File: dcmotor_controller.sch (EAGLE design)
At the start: 72 parts, among them IC1 L298, IC2 L298, IC3 AS5040, IC5 SN74LVCR162245A, Q1 8MHz, U1 STM32F051C8T6

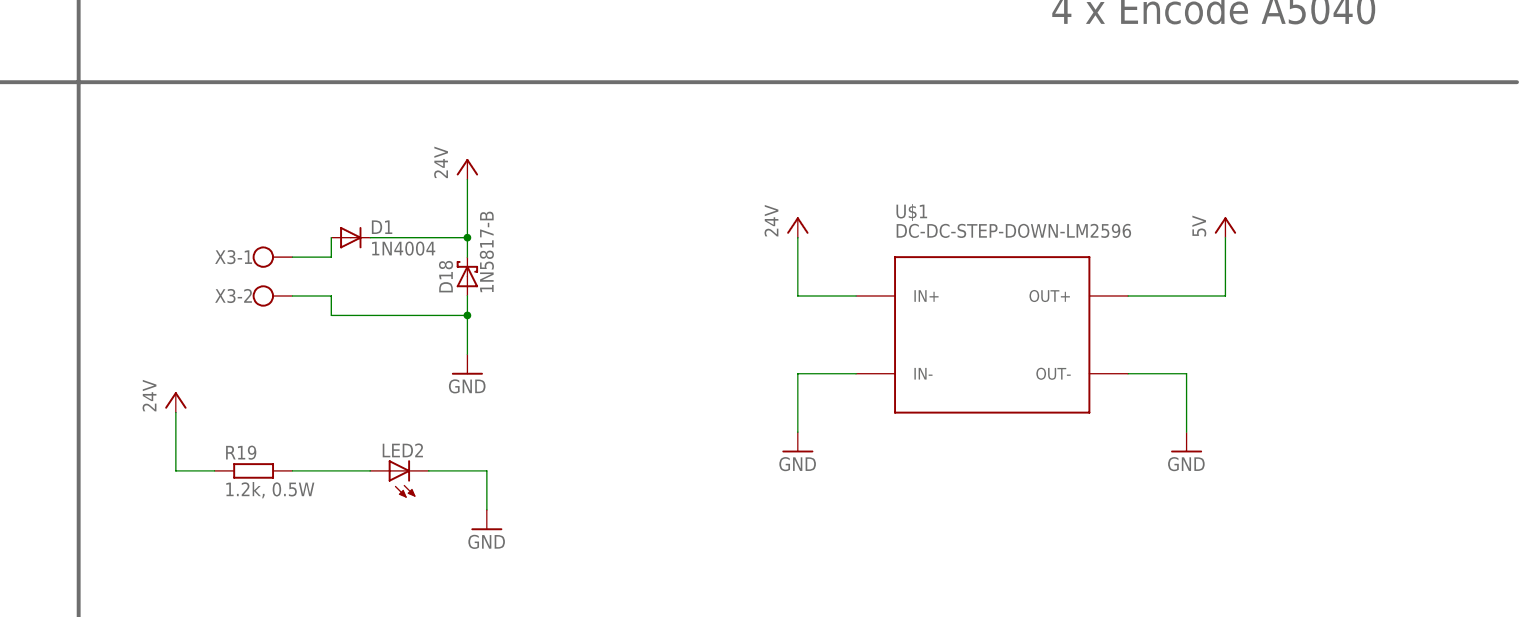
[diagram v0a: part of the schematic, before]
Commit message: poprawione zasilanie
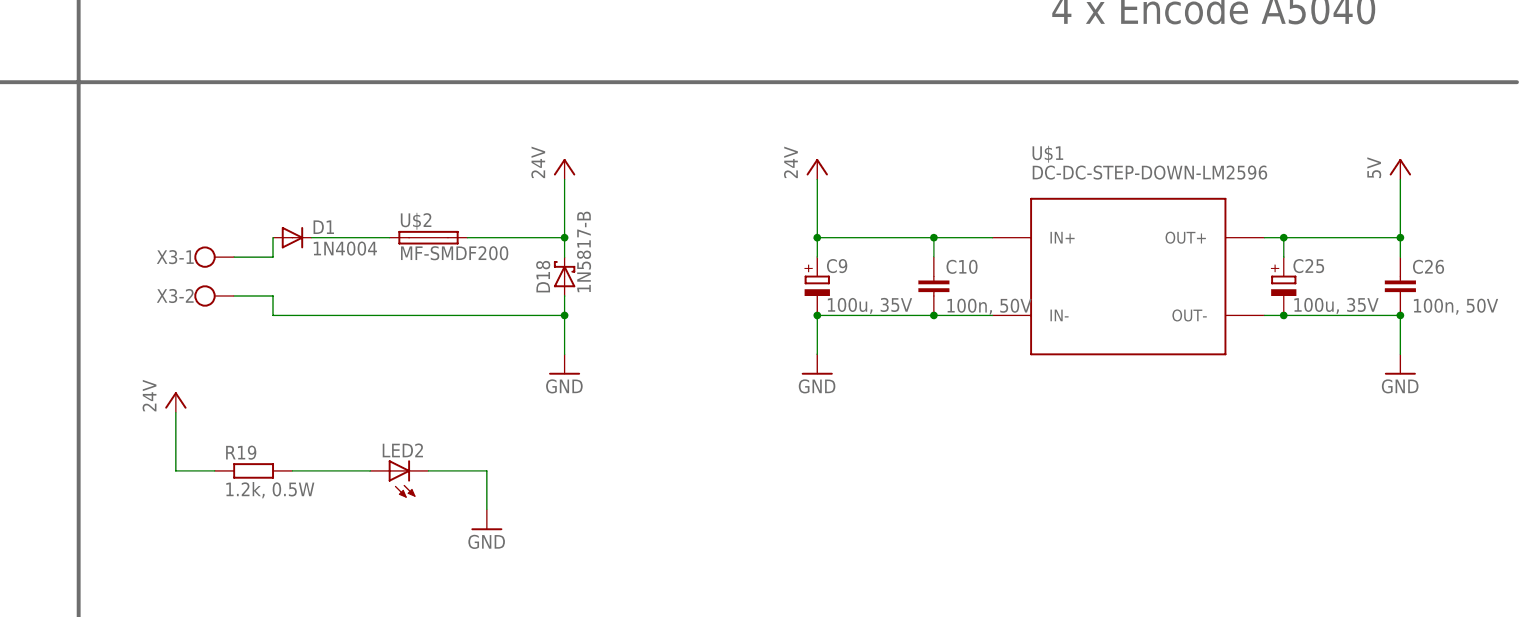
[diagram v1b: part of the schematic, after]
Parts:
- added C10, C26: 100n, 50V, rcl:C-EU025-025X050
- added C25, C9: 100u, 35V, rcl:CPOL-EUD
- added U$2: MF-SMDF200, fuse:MF-SMDF200
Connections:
- new net N$12: D1.C, U$2.1
- net GND: now also C10.2, C25.-, C26.2, C9.-
- net VCC: now also C10.1, C25.+, C26.1, C9.+, U$2.2; no longer D1.C
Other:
- moved on the sheet: D1, D18, U$1, X3-1, X3-2
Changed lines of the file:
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@@
 <part name="GND47" library="supply1" library_urn="urn:adsk.eagle:library:371" deviceset="GND" device=""/>
 <part name="P+5" library="supply1" library_urn="urn:adsk.eagle:library:371" deviceset="VCC" device="" value="5V"/>
+<part name="C9" library="rcl" library_urn="urn:adsk.eagle:library:334" deviceset="CPOL-EU" device="D" package3d_urn="urn:adsk.eagle:package:23424/2" value="100u, 35V"/>
+<part name="C10" library="rcl" library_urn="urn:adsk.eagle:library:334" deviceset="C-EU" device="025-025X050" package3d_urn="urn:adsk.eagle:package:23629/2" value="100n, 50V"/>
+<part name="C25" library="rcl" library_urn="urn:adsk.eagle:library:334" deviceset="CPOL-EU" device="D" package3d_urn="urn:adsk.eagle:package:23424/2" value="100u, 35V"/>
+<part name="C26" library="rcl" library_urn="urn:adsk.eagle:library:334" deviceset="C-EU" device="025-025X050" package3d_urn="urn:adsk.eagle:package:23629/2" value="100n, 50V"/>
+<part name="U$2" library="fuse" library_urn="urn:adsk.eagle:library:233" deviceset="MF-SMDF" device="" package3d_urn="urn:adsk.eagle:package:14081/1" technology="200"/>
 </parts>
 <sheets>
@@
 <instance part="GND43" gate="1" x="-353.06" y="76.2"/>
 <instance part="GND44" gate="1" x="-327.66" y="76.2"/>
-<instance part="D18" gate="G$1" x="-238.76" y="172.72" rot="R90"/>
-<instance part="X3" gate="-1" x="-266.7" y="175.26"/>
-<instance part="X3" gate="-2" x="-266.7" y="170.18"/>
-<instance part="P+11" gate="VCC" x="-238.76" y="187.96"/>
-<instance part="GND45" gate="1" x="-238.76" y="160.02"/>
+<instance part="D18" gate="G$1" x="-226.06" y="172.72" rot="R90"/>
+<instance part="X3" gate="-1" x="-274.32" y="175.26"/>
+<instance part="X3" gate="-2" x="-274.32" y="170.18"/>
+<instance part="P+11" gate="VCC" x="-226.06" y="187.96"/>
+<instance part="GND45" gate="1" x="-226.06" y="160.02"/>
 <instance part="P+12" gate="VCC" x="-276.86" y="157.48"/>
 <instance part="R19" gate="G$1" x="-266.7" y="147.32"/>
 <instance part="LED2" gate="G$1" x="-248.92" y="147.32" rot="R90"/>
 <instance part="GND46" gate="1" x="-236.22" y="139.7"/>
-<instance part="D1" gate="1" x="-254" y="177.8"/>
-<instance part="U$1" gate="G$1" x="-170.18" y="165.1"/>
-<instance part="P+4" gate="VCC" x="-195.58" y="180.34"/>
-<instance part="GND8" gate="1" x="-195.58" y="149.86"/>
-<instance part="GND47" gate="1" x="-144.78" y="149.86"/>
-<instance part="P+5" gate="VCC" x="-139.7" y="180.34"/>
+<instance part="D1" gate="1" x="-261.62" y="177.8"/>
+<instance part="U$1" gate="G$1" x="-152.4" y="172.72"/>
+<instance part="P+4" gate="VCC" x="-193.04" y="187.96"/>
+<instance part="GND8" gate="1" x="-193.04" y="160.02"/>
+<instance part="GND47" gate="1" x="-116.84" y="160.02"/>
+<instance part="P+5" gate="VCC" x="-116.84" y="187.96"/>
+<instance part="C9" gate="G$1" x="-193.04" y="172.72"/>
+<instance part="C10" gate="G$1" x="-177.8" y="172.72"/>
+<instance part="C25" gate="G$1" x="-132.08" y="172.72"/>
+<instance part="C26" gate="G$1" x="-116.84" y="172.72"/>
+<instance part="U$2" gate="A" x="-243.84" y="177.8"/>
 </instances>
 <busses>
@@
 <pinref part="GND45" gate="1" pin="GND"/>
 <pinref part="D18" gate="G$1" pin="A"/>
-<wire x1="-238.76" y1="170.18" x2="-238.76" y2="167.64" width="0.1524" layer="91"/>
+<wire x1="-226.06" y1="170.18" x2="-226.06" y2="167.64" width="0.1524" layer="91"/>
 <pinref part="X3" gate="-2" pin="KL"/>
-<wire x1="-238.76" y1="167.64" x2="-238.76" y2="162.56" width="0.1524" layer="91"/>
-<wire x1="-261.62" y1="170.18" x2="-256.54" y2="170.18" width="0.1524" layer="91"/>
-<wire x1="-256.54" y1="170.18" x2="-256.54" y2="167.64" width="0.1524" layer="91"/>
-<wire x1="-256.54" y1="167.64" x2="-238.76" y2="167.64" width="0.1524" layer="91"/>
-<junction x="-238.76" y="167.64"/>
+<wire x1="-226.06" y1="167.64" x2="-226.06" y2="162.56" width="0.1524" layer="91"/>
+<wire x1="-269.24" y1="170.18" x2="-264.16" y2="170.18" width="0.1524" layer="91"/>
+<wire x1="-264.16" y1="170.18" x2="-264.16" y2="167.64" width="0.1524" layer="91"/>
+<wire x1="-264.16" y1="167.64" x2="-226.06" y2="167.64" width="0.1524" layer="91"/>
+<junction x="-226.06" y="167.64"/>
 </segment>
 <segment>
@@
 <segment>
 <pinref part="U$1" gate="G$1" pin="IN-"/>
-<wire x1="-187.96" y1="160.02" x2="-195.58" y2="160.02" width="0.1524" layer="91"/>
-<wire x1="-195.58" y1="160.02" x2="-195.58" y2="152.4" width="0.1524" layer="91"/>
+<wire x1="-170.18" y1="167.64" x2="-177.8" y2="167.64" width="0.1524" layer="91"/>
+<wire x1="-177.8" y1="167.64" x2="-193.04" y2="167.64" width="0.1524" layer="91"/>
+<wire x1="-193.04" y1="167.64" x2="-193.04" y2="162.56" width="0.1524" layer="91"/>
 <pinref part="GND8" gate="1" pin="GND"/>
+<pinref part="C9" gate="G$1" pin="-"/>
+<junction x="-193.04" y="167.64"/>
+<pinref part="C10" gate="G$1" pin="2"/>
+<junction x="-177.8" y="167.64"/>
 </segment>
 <segment>
 <pinref part="U$1" gate="G$1" pin="OUT-"/>
-<wire x1="-152.4" y1="160.02" x2="-144.78" y2="160.02" width="0.1524" layer="91"/>
-<wire x1="-144.78" y1="160.02" x2="-144.78" y2="152.4" width="0.1524" layer="91"/>
+<wire x1="-134.62" y1="167.64" x2="-132.08" y2="167.64" width="0.1524" layer="91"/>
+<wire x1="-132.08" y1="167.64" x2="-116.84" y2="167.64" width="0.1524" layer="91"/>
+<wire x1="-116.84" y1="167.64" x2="-116.84" y2="162.56" width="0.1524" layer="91"/>
 <pinref part="GND47" gate="1" pin="GND"/>
+<pinref part="C25" gate="G$1" pin="-"/>
+<junction x="-132.08" y="167.64"/>
+<pinref part="C26" gate="G$1" pin="2"/>
+<junction x="-116.84" y="167.64"/>
 </segment>
 </net>
@@
 </segment>
 <segment>
-<wire x1="-251.46" y1="177.8" x2="-238.76" y2="177.8" width="0.1524" layer="91"/>
 <pinref part="D18" gate="G$1" pin="C"/>
-<wire x1="-238.76" y1="177.8" x2="-238.76" y2="175.26" width="0.1524" layer="91"/>
-<pinref part="D1" gate="1" pin="C"/>
 <pinref part="P+11" gate="VCC" pin="VCC"/>
-<wire x1="-238.76" y1="177.8" x2="-238.76" y2="185.42" width="0.1524" layer="91"/>
-<junction x="-238.76" y="177.8"/>
+<wire x1="-226.06" y1="175.26" x2="-226.06" y2="177.8" width="0.1524" layer="91"/>
+<pinref part="U$2" gate="A" pin="2"/>
+<wire x1="-226.06" y1="177.8" x2="-226.06" y2="185.42" width="0.1524" layer="91"/>
+<wire x1="-238.76" y1="177.8" x2="-226.06" y2="177.8" width="0.1524" layer="91"/>
+<junction x="-226.06" y="177.8"/>
 </segment>
 <segment>
 <pinref part="U$1" gate="G$1" pin="IN+"/>
-<wire x1="-187.96" y1="170.18" x2="-195.58" y2="170.18" width="0.1524" layer="91"/>
-<wire x1="-195.58" y1="170.18" x2="-195.58" y2="177.8" width="0.1524" layer="91"/>
+<wire x1="-170.18" y1="177.8" x2="-177.8" y2="177.8" width="0.1524" layer="91"/>
+<wire x1="-177.8" y1="177.8" x2="-193.04" y2="177.8" width="0.1524" layer="91"/>
+<wire x1="-193.04" y1="177.8" x2="-193.04" y2="185.42" width="0.1524" layer="91"/>
 <pinref part="P+4" gate="VCC" pin="VCC"/>
+<pinref part="C9" gate="G$1" pin="+"/>
+<wire x1="-193.04" y1="175.26" x2="-193.04" y2="177.8" width="0.1524" layer="91"/>
+<junction x="-193.04" y="177.8"/>
+<pinref part="C10" gate="G$1" pin="1"/>
+<wire x1="-177.8" y1="175.26" x2="-177.8" y2="177.8" width="0.1524" layer="91"/>
+<junction x="-177.8" y="177.8"/>
 </segment>
 <segment>
 <pinref part="U$1" gate="G$1" pin="OUT+"/>
-<wire x1="-152.4" y1="170.18" x2="-139.7" y2="170.18" width="0.1524" layer="91"/>
-<wire x1="-139.7" y1="170.18" x2="-139.7" y2="177.8" width="0.1524" layer="91"/>
+<wire x1="-134.62" y1="177.8" x2="-132.08" y2="177.8" width="0.1524" layer="91"/>
+<wire x1="-132.08" y1="177.8" x2="-116.84" y2="177.8" width="0.1524" layer="91"/>
+<wire x1="-116.84" y1="177.8" x2="-116.84" y2="185.42" width="0.1524" layer="91"/>
 <pinref part="P+5" gate="VCC" pin="VCC"/>
+<pinref part="C25" gate="G$1" pin="+"/>
+<wire x1="-132.08" y1="175.26" x2="-132.08" y2="177.8" width="0.1524" layer="91"/>
+<junction x="-132.08" y="177.8"/>
+<pinref part="C26" gate="G$1" pin="1"/>
+<wire x1="-116.84" y1="175.26" x2="-116.84" y2="177.8" width="0.1524" layer="91"/>
+<junction x="-116.84" y="177.8"/>
 </segment>
 </net>
@@
 <segment>
 <pinref part="X3" gate="-1" pin="KL"/>
-<wire x1="-261.62" y1="175.26" x2="-256.54" y2="175.26" width="0.1524" layer="91"/>
-<wire x1="-256.54" y1="175.26" x2="-256.54" y2="177.8" width="0.1524" layer="91"/>
+<wire x1="-269.24" y1="175.26" x2="-264.16" y2="175.26" width="0.1524" layer="91"/>
+<wire x1="-264.16" y1="175.26" x2="-264.16" y2="177.8" width="0.1524" layer="91"/>
 <pinref part="D1" gate="1" pin="A"/>
 </segment>
 </net>
+<net name="N$12" class="0">
+<segment>
+<pinref part="D1" gate="1" pin="C"/>
+<pinref part="U$2" gate="A" pin="1"/>
+<wire x1="-259.08" y1="177.8" x2="-248.92" y2="177.8" width="0.1524" layer="91"/>
+</segment>
+</net>
